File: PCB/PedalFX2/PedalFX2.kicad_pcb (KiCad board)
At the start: 2 copper layers, 55.5 x 42.5 mm, 12 parts, among them J1 Conn_01x04_Female, T1 ACJS-MHDR, T2 ACJS-MHDR, T3 54-00129

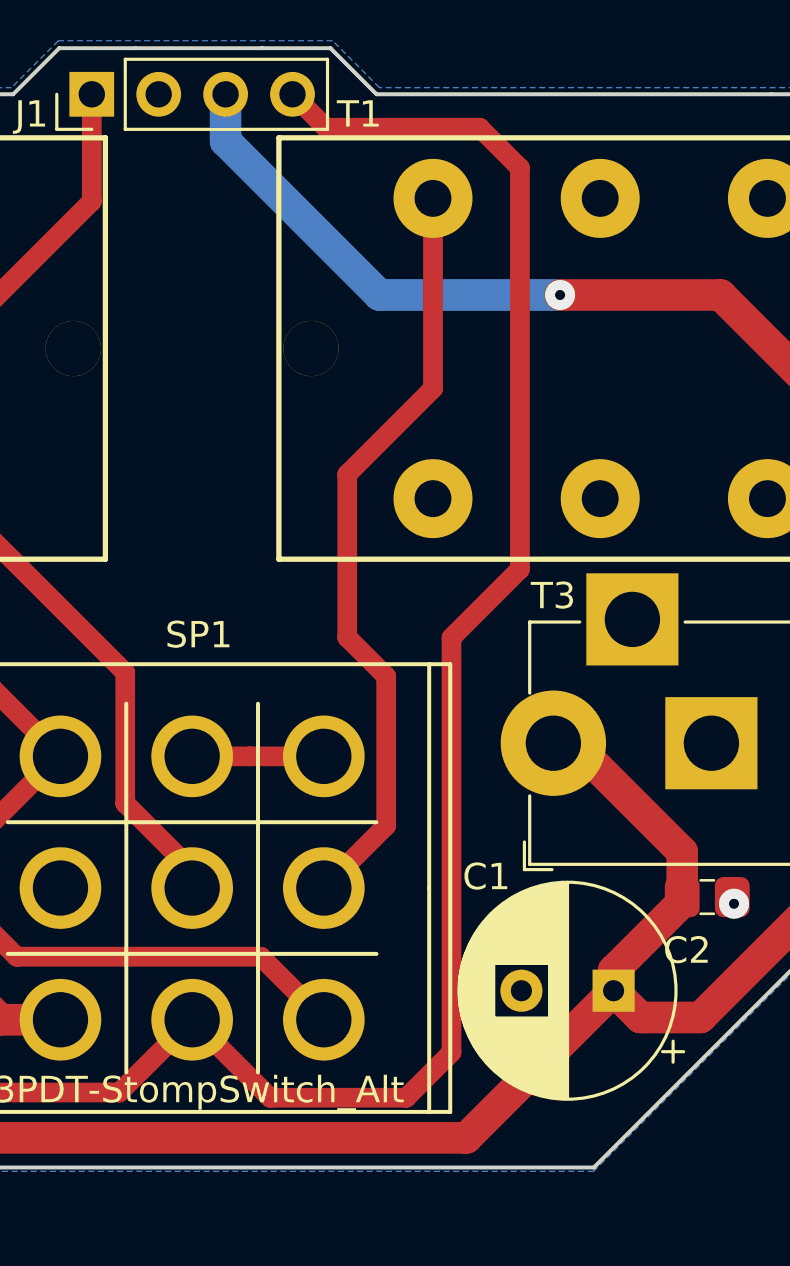
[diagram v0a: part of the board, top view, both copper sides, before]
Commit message: Minor Tweaks
Minor tweaks to PCB
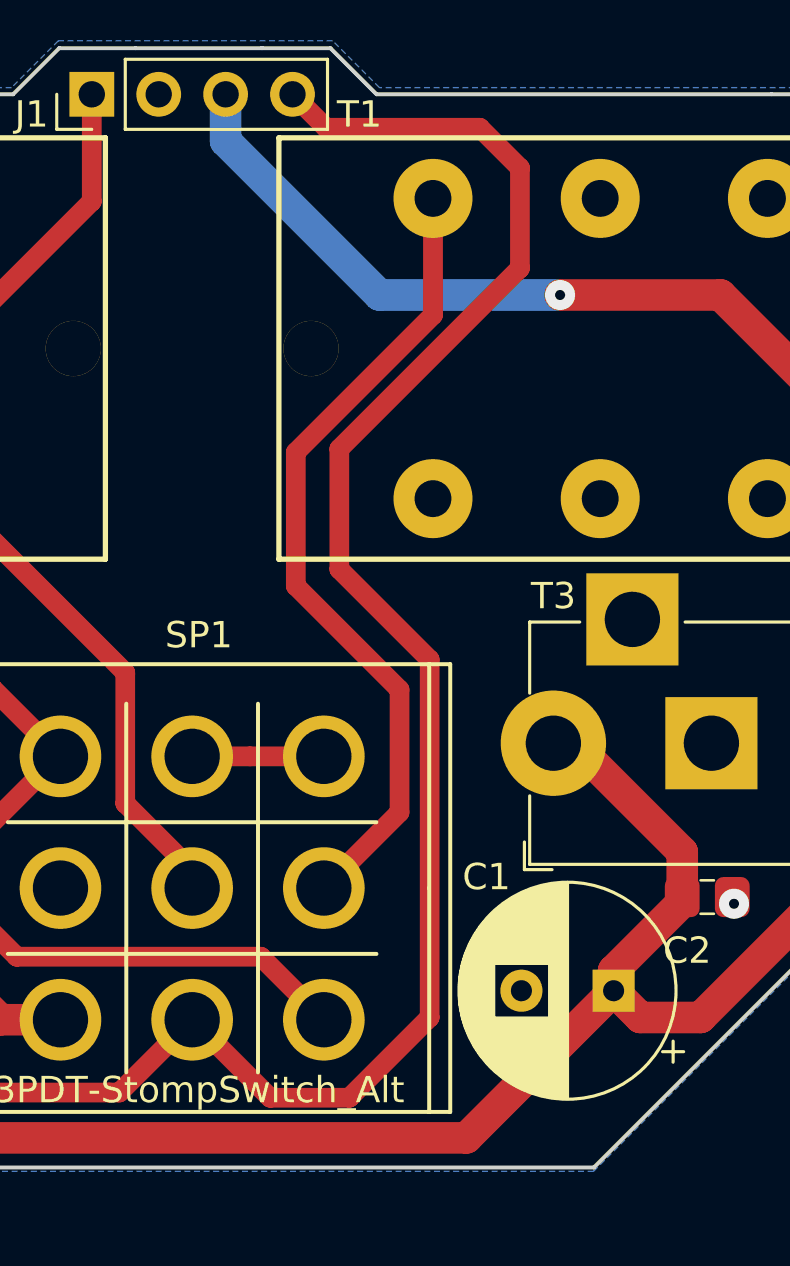
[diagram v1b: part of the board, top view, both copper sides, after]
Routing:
- net Net-(SP1-Pad4): track 29.1 -> 31.2 mm
- net Net-(J1-Pad4): track 68.8 -> 70.4 mm
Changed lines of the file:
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@@
     (thickness 1.6)
     (drawings 20)
-    (tracks 73)
+    (tracks 75)
     (zones 0)
     (modules 12)
@@
     (solder_mask_min_width 0.25)
     (aux_axis_origin 0 0)
-    (visible_elements FFFFFF7F)
+    (visible_elements 7FFFFFFF)
     (pcbplotparams
       (layerselection 0x010fc_ffffffff)
@@
   (segment (start 145.288 109.982) (end 138.43 109.982) (width 1.2) (layer B.Cu) (net 2))
   (segment (start 138.43 109.982) (end 132.588 104.14) (width 1.2) (layer B.Cu) (net 2))
-  (segment (start 136.398 103.632) (end 135.128 102.362) (width 0.75) (layer F.Cu) (net 3))
-  (segment (start 142.24 103.632) (end 136.398 103.632) (width 0.75) (layer F.Cu) (net 3))
-  (segment (start 143.764 105.156) (end 142.24 103.632) (width 0.75) (layer F.Cu) (net 3))
-  (segment (start 134.28 140.462) (end 139.446 140.462) (width 0.75) (layer F.Cu) (net 3))
-  (segment (start 139.446 140.462) (end 141.166501 138.741499) (width 0.75) (layer F.Cu) (net 3))
-  (segment (start 131.318 137.5) (end 134.28 140.462) (width 0.75) (layer F.Cu) (net 3))
-  (segment (start 141.166501 138.741499) (end 141.166501 122.993499) (width 0.75) (layer F.Cu) (net 3))
-  (segment (start 141.166501 122.993499) (end 143.764 120.396) (width 0.75) (layer F.Cu) (net 3))
-  (segment (start 143.764 120.396) (end 143.764 105.156) (width 0.75) (layer F.Cu) (net 3))
   (segment (start 128.157 140.263) (end 119.888 140.263) (width 0.75) (layer F.Cu) (net 3))
   (segment (start 131.318 137.5) (end 128.555 140.263) (width 0.75) (layer F.Cu) (net 3))
   (segment (start 128.555 140.263) (end 128.157 140.263) (width 0.75) (layer F.Cu) (net 3))
+  (segment (start 136.398 103.632) (end 135.128 102.362) (width 0.75) (layer F.Cu) (net 3))
+  (segment (start 143.764 105.156) (end 142.24 103.632) (width 0.75) (layer F.Cu) (net 3))
+  (segment (start 137.287 140.462) (end 140.335 137.414) (width 0.75) (layer F.Cu) (net 3))
+  (segment (start 134.28 140.462) (end 137.287 140.462) (width 0.75) (layer F.Cu) (net 3))
+  (segment (start 140.335 137.414) (end 140.335 123.825) (width 0.75) (layer F.Cu) (net 3))
+  (segment (start 142.24 103.632) (end 136.398 103.632) (width 0.75) (layer F.Cu) (net 3))
+  (segment (start 131.318 137.5) (end 134.28 140.462) (width 0.75) (layer F.Cu) (net 3))
+  (segment (start 143.764 108.966) (end 143.764 105.156) (width 0.75) (layer F.Cu) (net 3))
+  (segment (start 136.906 115.824) (end 143.764 108.966) (width 0.75) (layer F.Cu) (net 3))
+  (segment (start 140.335 123.825) (end 136.906 120.396) (width 0.75) (layer F.Cu) (net 3))
+  (segment (start 136.906 120.396) (end 136.906 115.824) (width 0.75) (layer F.Cu) (net 3))
   (segment (start 126.238 127.42) (end 126.318 127.5) (width 0.25) (layer F.Cu) (net 4))
   (segment (start 126.318 128.858) (end 126.318 127.5) (width 0.25) (layer F.Cu) (net 4))
@@
   (segment (start 126.318 137.5) (end 124.038 137.5) (width 1.2) (layer F.Cu) (net 6))
   (segment (start 124.038 137.5) (end 120.396 133.858) (width 1.2) (layer F.Cu) (net 6))
-  (segment (start 137.207001 122.983001) (end 137.207001 116.792999) (width 0.75) (layer F.Cu) (net 7))
-  (segment (start 138.684 124.46) (end 137.207001 122.983001) (width 0.75) (layer F.Cu) (net 7))
-  (segment (start 137.207001 116.792999) (end 140.462 113.538) (width 0.75) (layer F.Cu) (net 7))
-  (segment (start 140.462 113.538) (end 140.462 106.314) (width 0.75) (layer F.Cu) (net 7))
-  (segment (start 138.684 130.134) (end 138.684 124.46) (width 0.75) (layer F.Cu) (net 7))
-  (segment (start 136.318 132.5) (end 138.684 130.134) (width 0.75) (layer F.Cu) (net 7))
+  (segment (start 136.318 132.5) (end 139.192 129.626) (width 0.75) (layer F.Cu) (net 7))
+  (segment (start 140.462 110.744) (end 140.462 106.314) (width 0.75) (layer F.Cu) (net 7))
+  (segment (start 135.255 115.951) (end 140.462 110.744) (width 0.75) (layer F.Cu) (net 7))
+  (segment (start 135.255 121.031) (end 135.255 115.951) (width 0.75) (layer F.Cu) (net 7))
+  (segment (start 139.192 124.968) (end 135.255 121.031) (width 0.75) (layer F.Cu) (net 7))
+  (segment (start 139.192 129.626) (end 139.192 124.968) (width 0.75) (layer F.Cu) (net 7))
   (segment (start 128.778 124.318) (end 122.174 117.714) (width 0.75) (layer F.Cu) (net 8))
   (segment (start 128.778 129.286) (end 128.778 124.318) (width 0.75) (layer F.Cu) (net 8))
